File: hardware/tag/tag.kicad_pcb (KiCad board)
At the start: 2 copper layers, 94 x 45.7 mm, 8 parts

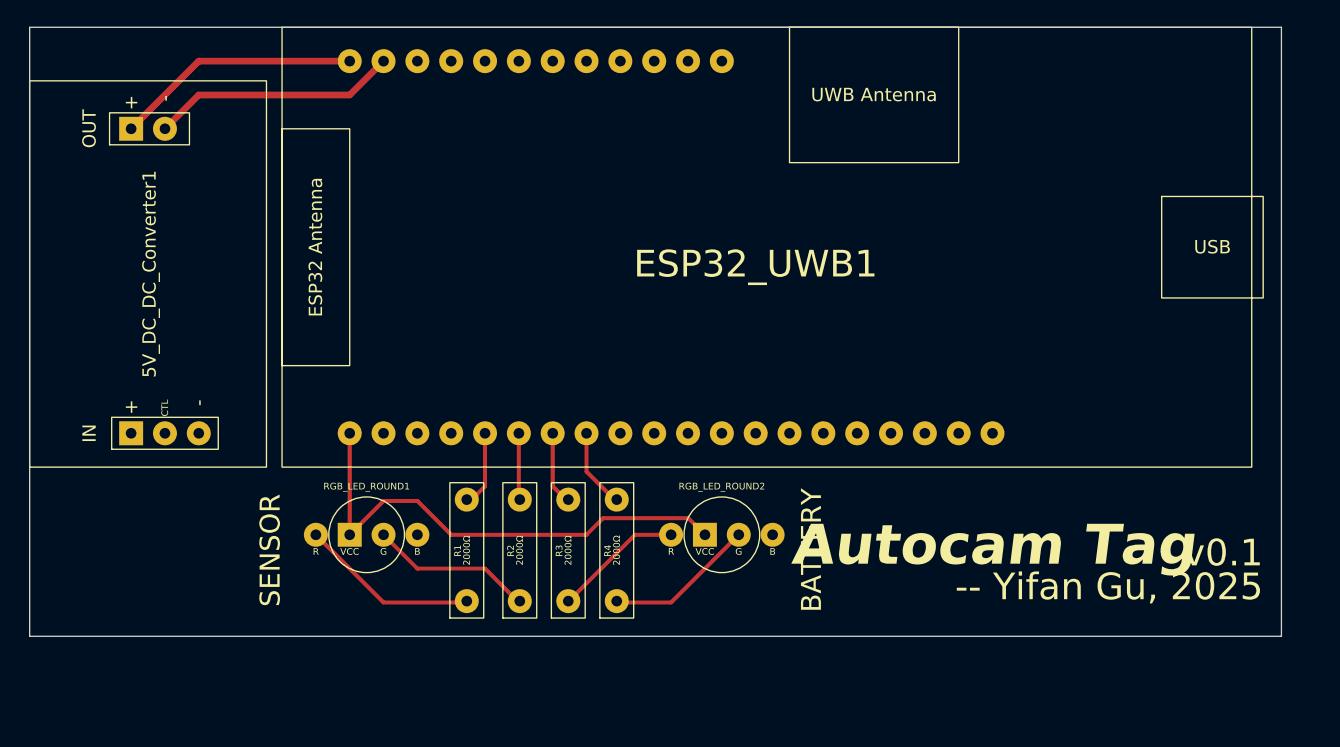
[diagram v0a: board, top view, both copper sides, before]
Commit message: hardware: Add remote PCB.
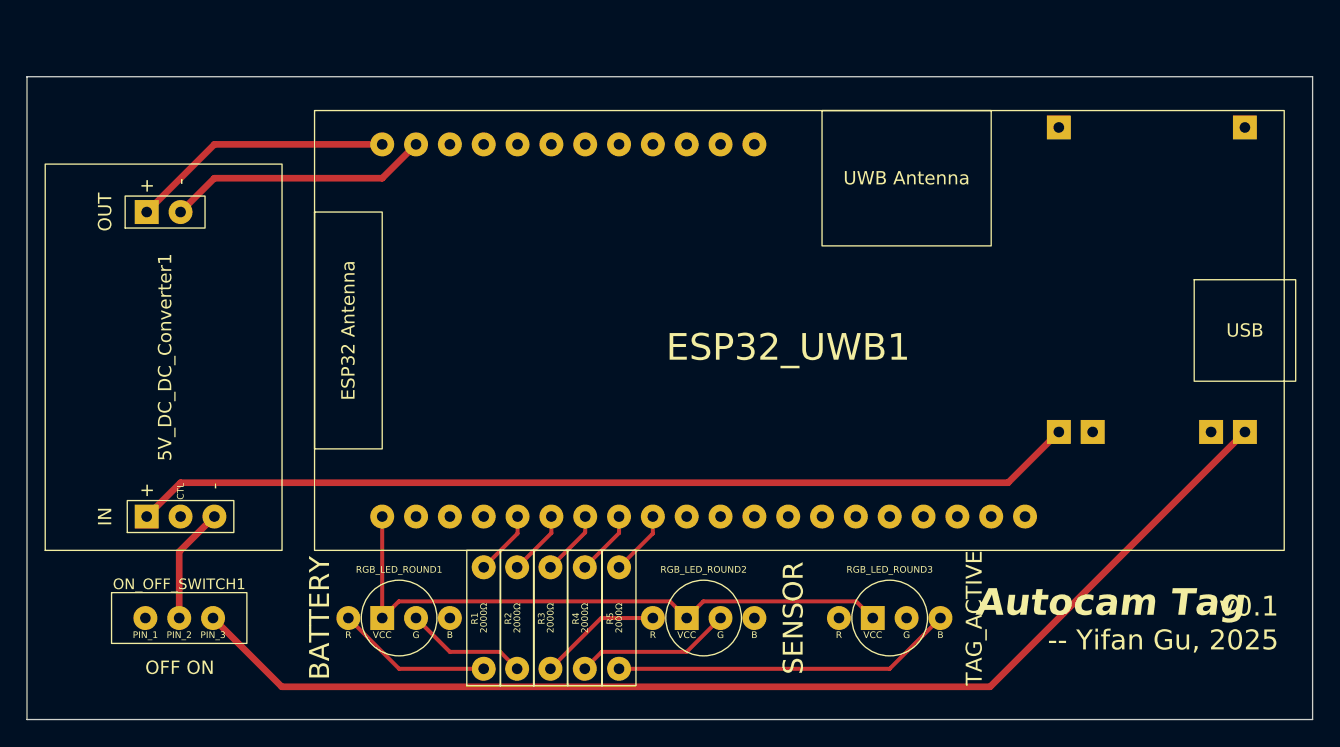
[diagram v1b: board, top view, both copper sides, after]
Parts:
- added Battery_Charger1: ~, Autocam:USB-C 3.7V Lithium Battery Charger, B.Cu at (192.2, 78.7)
- added ON_OFF_SWITCH1: OFF ON, Autocam:3-PIN Switch, F.Cu at (108.0, 116.8)
- added R5: 2000Ω, Autocam:Simple Resistor, F.Cu at (143.5, 120.7)
- added RGB_LED_ROUND3: TAG_ACTIVE, Autocam:Anode RGB LED (Round), F.Cu at (163.8, 116.8)
- RGB_LED_ROUND1: value SENSOR -> BATTERY
- RGB_LED_ROUND2: value BATTERY -> SENSOR
- moved ESP32_UWB1 6.71 mm to (120.7, 78.7)
- moved RGB_LED_ROUND1 6.71 mm to (127.0, 116.8)
- moved RGB_LED_ROUND2 6.40 mm to (149.9, 116.8)
- moved 5V_DC_DC_Converter1 6.36 mm to (100.4, 111.8)
- moved R4 5.62 mm to (140.9, 120.7)
- moved R3 5.25 mm to (138.4, 120.7)
- moved R1 5.24 mm to (133.3, 120.7)
- moved R2 5.08 mm to (135.9, 120.7)
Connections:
- 5V_DC_DC_Converter1 pad 1: unconnected-(5V_DC_DC_Converter1-+-Pad1) -> Net-(Battery_Charger1-OUT+)
- 5V_DC_DC_Converter1 pad 3: unconnected-(5V_DC_DC_Converter1---Pad3) -> Net-(5V_DC_DC_Converter1---Pad3)
- ESP32_UWB1 pad 9: unconnected-(ESP32_UWB1-IO15-Pad9) -> Net-(ESP32_UWB1-IO15)
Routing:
- net Net-(Battery_Charger1-OUT-): track 0.00 -> 87.5 mm
- net Net-(Battery_Charger1-OUT+): track 0.00 -> 71.1 mm
- net Net-(RGB_LED_ROUND3-B): track 0.00 -> 25.7 mm
- net Net-(ESP32_UWB1-3V3): track 37.4 -> 46.5 mm
- net Net-(5V_DC_DC_Converter1---Pad3): track 0.00 -> 8.71 mm
- net Net-(ESP32_UWB1-IO15): track 0.00 -> 4.90 mm
- net Net-(RGB_LED_ROUND1-G): track 12.3 -> 9.17 mm
- net Net-(RGB_LED_ROUND1-R): track 13.7 -> 11.7 mm
- net Net-(5V_DC_DC_Converter1---Pad5): track 18.5 -> 19.8 mm
- net Net-(ESP32_UWB1-5V0): track 18.5 -> 19.8 mm
- net Net-(ESP32_UWB1-IO14): track 6.50 -> 5.48 mm
- net Net-(ESP32_UWB1-IO2): track 5.54 -> 4.86 mm
- net Net-(RGB_LED_ROUND2-R): track 9.89 -> 9.27 mm
- net Net-(ESP32_UWB1-IO13): track 5.54 -> 4.93 mm
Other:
- board size 94 x 45.7 mm -> 96.5 x 48.3 mm
